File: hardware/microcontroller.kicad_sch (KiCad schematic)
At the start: 5 parts

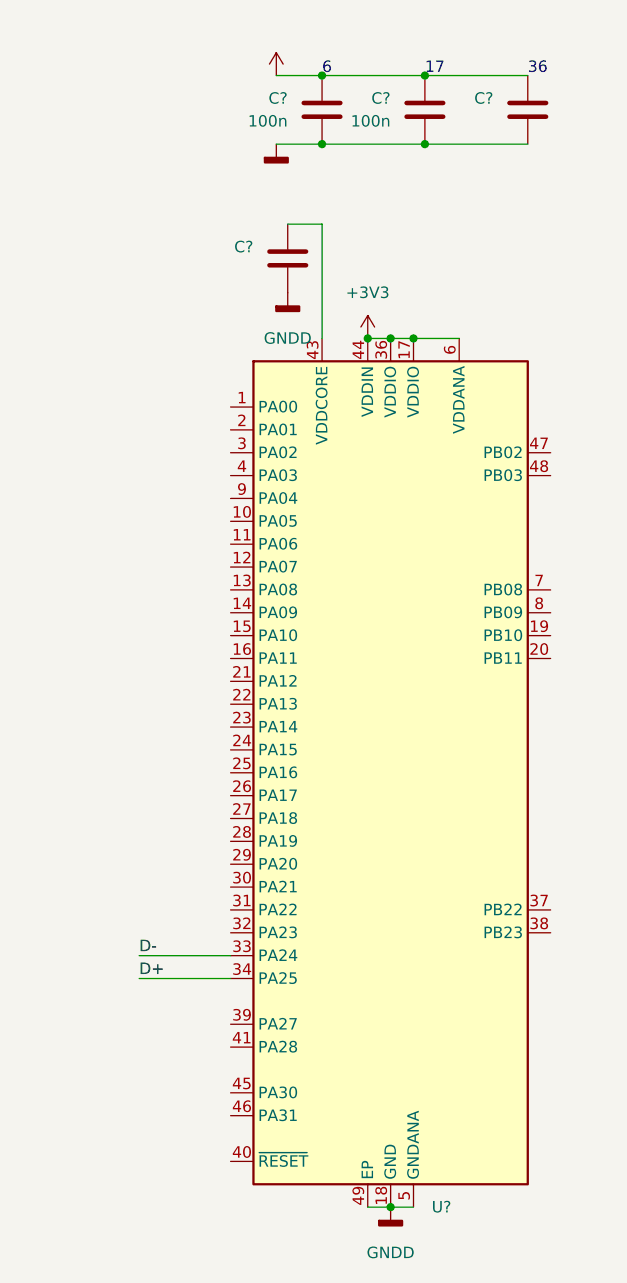
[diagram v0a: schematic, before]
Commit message: Version 1 of driver and current sense.
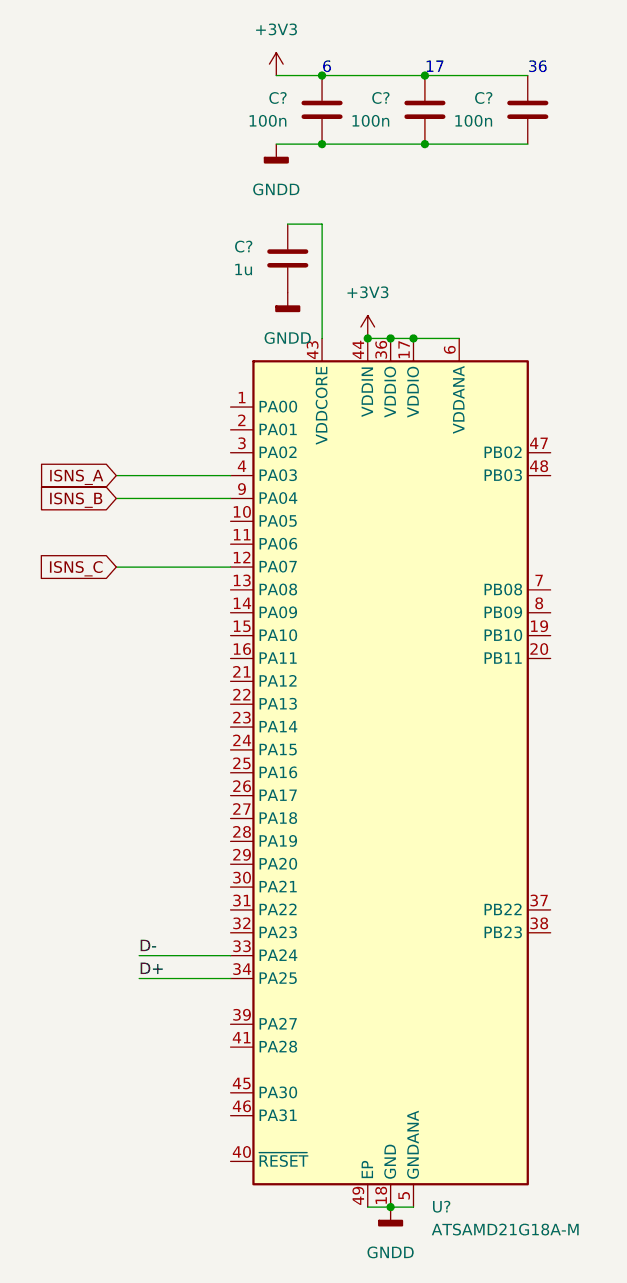
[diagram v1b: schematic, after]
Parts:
- C?: value (none) -> 1u; footprint (none) -> Capacitor_SMD:C_0402_1005Metric
- C?: value (none) -> 100n; footprint (none) -> Capacitor_SMD:C_0402_1005Metric
- U?: value (none) -> ATSAMD21G18A-M; footprint (none) -> Package_DFN_QFN:QFN-48-1EP_7x7mm_P0.5mm_EP5.15x5.15mm
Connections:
- net ISNS_C: now reaches U?.12 (PA07)
- net ISNS_A: now reaches U?.4 (PA03)
- net ISNS_B: now reaches U?.9 (PA04)
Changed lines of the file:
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@@
+    (stroke (width 0) (type default) (color 0 0 0 0))
+  )
+  (wire (pts (xy 109.22 68.58) (xy 121.92 68.58))
     (stroke (width 0) (type default) (color 0 0 0 0))
   )
@@
     (stroke (width 0) (type default) (color 0 0 0 0))
   )
+  (wire (pts (xy 109.22 71.12) (xy 121.92 71.12))
+    (stroke (width 0) (type default) (color 0 0 0 0))
+  )
   (wire (pts (xy 132.08 24.13) (xy 143.51 24.13))
     (stroke (width 0) (type default) (color 0 0 0 0))
@@
     (stroke (width 0) (type default) (color 0 0 0 0))
   )
+  (wire (pts (xy 109.22 78.74) (xy 121.92 78.74))
+    (stroke (width 0) (type default) (color 0 0 0 0))
+  )
   (wire (pts (xy 111.76 121.92) (xy 121.92 121.92))
     (stroke (width 0) (type default) (color 0 0 0 0))
@@
     (effects (font (size 1.27 1.27)) (justify left bottom))
   )
+  (global_label "ISNS_C" (shape input) (at 109.22 78.74 180) (fields_autoplaced)
+    (effects (font (size 1.27 1.27)) (justify right))
+    (property "Intersheet References" "${INTERSHEET_REFS}" (id 0) (at 100.215 78.6606 0)
+      (effects (font (size 1.27 1.27)) (justify right) hide)
+    )
+  )
+  (global_label "ISNS_A" (shape input) (at 109.22 68.58 180) (fields_autoplaced)
+    (effects (font (size 1.27 1.27)) (justify right))
+    (property "Intersheet References" "${INTERSHEET_REFS}" (id 0) (at 100.3964 68.5006 0)
+      (effects (font (size 1.27 1.27)) (justify right) hide)
+    )
+  )
+  (global_label "ISNS_B" (shape input) (at 109.22 71.12 180) (fields_autoplaced)
+    (effects (font (size 1.27 1.27)) (justify right))
+    (property "Intersheet References" "${INTERSHEET_REFS}" (id 0) (at 100.215 71.0406 0)
+      (effects (font (size 1.27 1.27)) (justify right) hide)
+    )
+  )
   (symbol (lib_id "power:+3V3") (at 127 24.13 0) (unit 1)
     (in_bom yes) (on_board yes) (fields_autoplaced)
@@
       (effects (font (size 1.27 1.27)) hide)
     )
-    (property "Value" "" (id 1) (at 127 19.05 0))
+    (property "Value" "+3V3" (id 1) (at 127 19.05 0))
     (property "Footprint" "" (id 2) (at 127 24.13 0)
       (effects (font (size 1.27 1.27)) hide)
@@
       (effects (font (size 1.27 1.27)) hide)
     )
-    (property "Value" "" (id 1) (at 127 36.83 0))
+    (property "Value" "GNDD" (id 1) (at 127 36.83 0))
     (property "Footprint" "" (id 2) (at 127 31.75 0)
       (effects (font (size 1.27 1.27)) hide)
@@
       (effects (font (size 1.27 1.27)) (justify right))
     )
-    (property "Value" "" (id 1) (at 124.46 45.7199 0)
-      (effects (font (size 1.27 1.27)) (justify right))
-    )
-    (property "Footprint" "" (id 2) (at 129.2352 40.64 0)
+    (property "Value" "1u" (id 1) (at 124.46 45.7199 0)
+      (effects (font (size 1.27 1.27)) (justify right))
+    )
+    (property "Footprint" "Capacitor_SMD:C_0402_1005Metric" (id 2) (at 129.2352 40.64 0)
       (effects (font (size 1.27 1.27)) hide)
     )
@@
       (effects (font (size 1.27 1.27)) (justify right))
     )
-    (property "Value" "" (id 1) (at 151.13 29.2099 0)
-      (effects (font (size 1.27 1.27)) (justify right))
-    )
-    (property "Footprint" "" (id 2) (at 155.9052 24.13 0)
+    (property "Value" "100n" (id 1) (at 151.13 29.2099 0)
+      (effects (font (size 1.27 1.27)) (justify right))
+    )
+    (property "Footprint" "Capacitor_SMD:C_0402_1005Metric" (id 2) (at 155.9052 24.13 0)
       (effects (font (size 1.27 1.27)) hide)
     )
@@
       (effects (font (size 1.27 1.27)) (justify left))
     )
-    (property "Value" "" (id 1) (at 144.2594 152.4 0)
+    (property "Value" "ATSAMD21G18A-M" (id 1) (at 144.2594 152.4 0)
       (effects (font (size 1.27 1.27)) (justify left))
     )
-    (property "Footprint" "" (id 2) (at 175.26 148.59 0)
-      (effects (font (size 1.27 1.27)) hide)
-    )
+    (property "Footprint" "Package_DFN_QFN:QFN-48-1EP_7x7mm_P0.5mm_EP5.15x5.15mm" (id 2) (at 175.26 148.59 0)
+      (effects (font (size 1.27 1.27)) hide)
+    )
